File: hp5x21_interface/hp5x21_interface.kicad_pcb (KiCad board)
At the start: 2 copper layers, 4 parts, among them IC1 74LVC4245APW,118, IC2 74LVC4245APW,118, IC3 74LVC4245APW,118

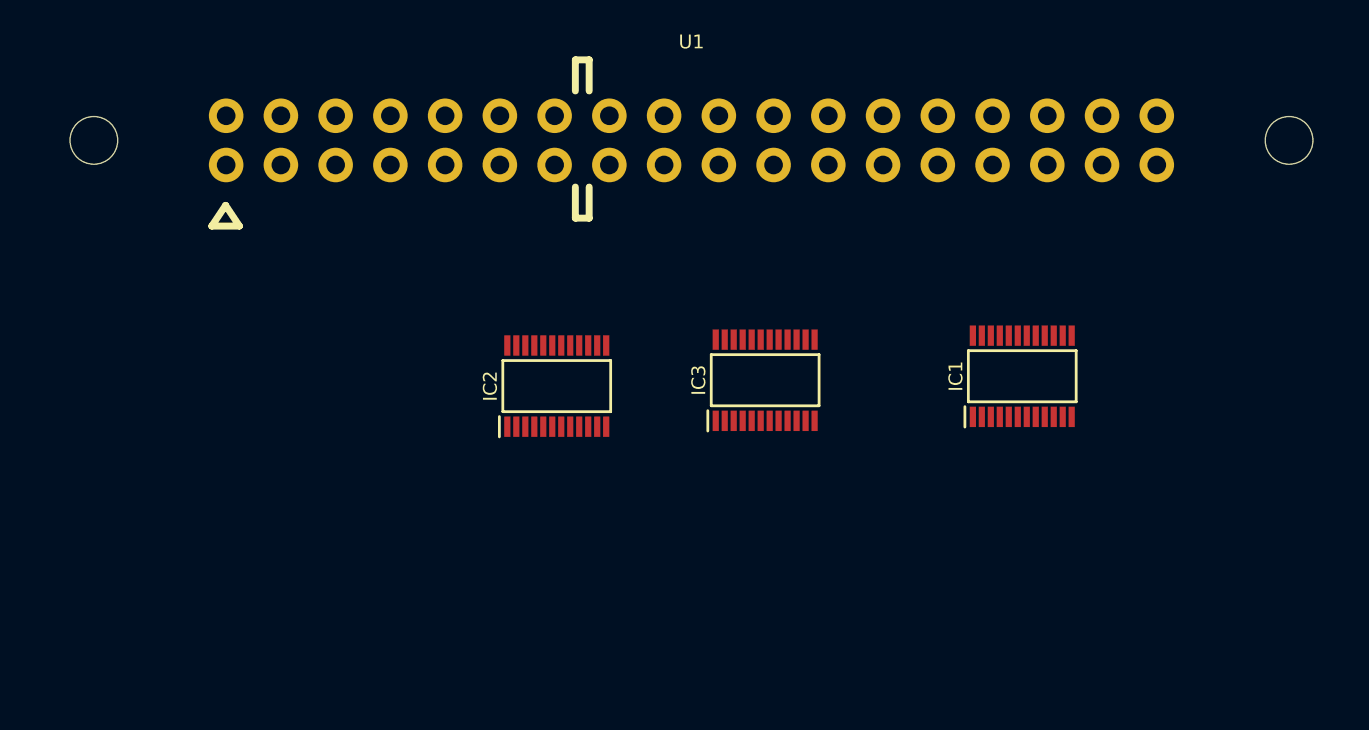
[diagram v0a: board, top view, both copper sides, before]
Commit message: Updated and released to JLCPCB
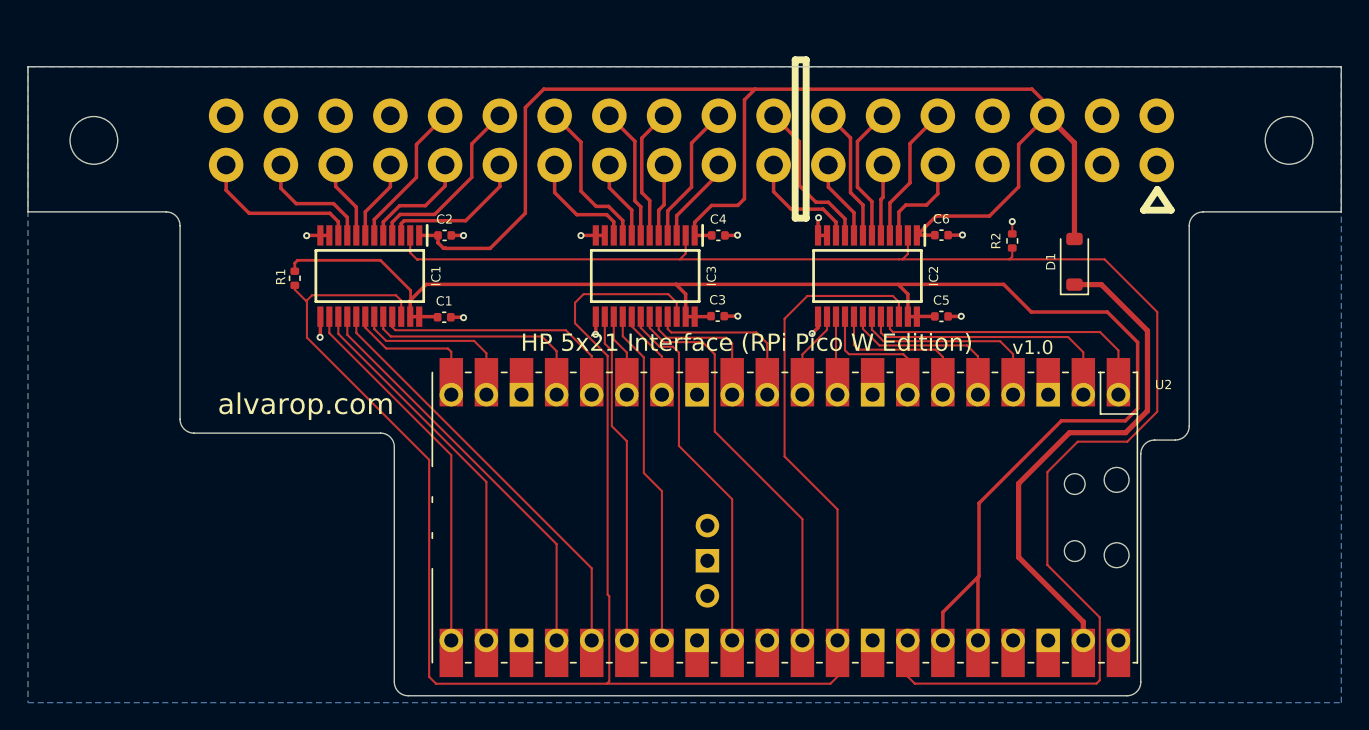
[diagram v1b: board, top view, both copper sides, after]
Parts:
- added C1: 0.1uF, Capacitor_SMD:C_0402_1005Metric, F.Cu at (120.1, 113.1)
- added C2: 0.1uF, Capacitor_SMD:C_0402_1005Metric, F.Cu at (120.1, 107.2)
- added C3: 0.1uF, Capacitor_SMD:C_0402_1005Metric, F.Cu at (139.9, 113.0)
- added C4: 0.1uF, Capacitor_SMD:C_0402_1005Metric, F.Cu at (139.9, 107.2)
- added C5: 0.1uF, Capacitor_SMD:C_0402_1005Metric, F.Cu at (156.1, 113.1)
- added C6: 0.1uF, Capacitor_SMD:C_0402_1005Metric, F.Cu at (156.1, 107.2)
- added D1: D_Schottky, Diode_SMD:D_SOD-123, F.Cu at (165.7, 109.1)
- added R1: 100k, Resistor_SMD:R_0402_1005Metric, F.Cu at (109.3, 110.3)
- added R2: 100k, Resistor_SMD:R_0402_1005Metric, F.Cu at (161.2, 107.6)
- added U2: PicoW, RP2040:RPi_PicoW_SMD_TH, F.Cu at (144.8, 127.6)
- U1: value ~ -> 307-036-520-201; moved to B.Cu
- moved IC1 47.8 mm to (114.7, 110.1), turned to -90 degrees
- moved IC2 23.8 mm to (150.7, 110.1), turned to -90 degrees
- moved IC3 11.5 mm to (134.7, 110.1), turned to -90 degrees
- turned U1 to 180 degrees
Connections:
- IC1 pad 1: unconnected-(IC1-VCC(A)-Pad1) -> +5V
- IC1 pad 10: unconnected-(IC1-A7-Pad10) -> /IO0_D
- IC1 pad 11: unconnected-(IC1-GND_1-Pad11) -> GND
- IC1 pad 12: unconnected-(IC1-GND_2-Pad12) -> GND
- IC1 pad 13: unconnected-(IC1-GND_3-Pad13) -> GND
- IC1 pad 14: /IO0_D -> /IO0_D_3V
- IC1 pad 15: /IO0_C -> /IO0_A_3V
- IC1 pad 16: /IO0_B -> /IO0_B_3V
- IC1 pad 17: /IO0_A -> /IO0_C_3V
- IC1 pad 18: /IO3_D -> /IO3_A_3V
- IC1 pad 19: /IO3_C -> /IO5_C_3V
- IC1 pad 2: unconnected-(IC1-DIR-Pad2) -> /DIR
- IC1 pad 20: /IO3_B -> /IO3_D_3V
- IC1 pad 21: /IO3_A -> /IO5_B_3V
- IC1 pad 22: unconnected-(IC1-~{OE}-Pad22) -> /~{OE}
- IC1 pad 23: unconnected-(IC1-VCC(B)_1-Pad23) -> +3.3V
- IC1 pad 24: unconnected-(IC1-VCC(B)_2-Pad24) -> +3.3V
- IC1 pad 3: unconnected-(IC1-A0-Pad3) -> /IO5_B
- IC1 pad 4: unconnected-(IC1-A1-Pad4) -> /IO3_D
- IC1 pad 5: unconnected-(IC1-A2-Pad5) -> /IO5_C
- IC1 pad 6: unconnected-(IC1-A3-Pad6) -> /IO3_A
- IC1 pad 7: unconnected-(IC1-A4-Pad7) -> /IO0_C
- IC1 pad 8: unconnected-(IC1-A5-Pad8) -> /IO0_B
- IC1 pad 9: unconnected-(IC1-A6-Pad9) -> /IO0_A
- IC2 pad 1: unconnected-(IC2-VCC(A)-Pad1) -> +5V
- IC2 pad 10: unconnected-(IC2-A7-Pad10) -> /IO1_C
- IC2 pad 11: unconnected-(IC2-GND_1-Pad11) -> GND
- IC2 pad 12: unconnected-(IC2-GND_2-Pad12) -> GND
- IC2 pad 13: unconnected-(IC2-GND_3-Pad13) -> GND
- IC2 pad 14: /IO2_D -> /IO1_C_3V
- IC2 pad 15: /IO2_C -> /IO2_C_3V
- IC2 pad 16: /IO2_B -> /IO1_B_3V
- IC2 pad 17: /IO2_A -> /IO2_B_3V
- IC2 pad 18: /IO1_D -> /IO2_A_3V
- IC2 pad 19: /IO1_C -> /IO1_A_3V
- IC2 pad 2: unconnected-(IC2-DIR-Pad2) -> /DIR
- IC2 pad 20: /IO1_B -> /IO2_D_3V
- IC2 pad 21: /IO1_A -> /IO1_D_3V
- IC2 pad 22: unconnected-(IC2-~{OE}-Pad22) -> /~{OE}
- IC2 pad 23: unconnected-(IC2-VCC(B)_1-Pad23) -> +3.3V
- IC2 pad 24: unconnected-(IC2-VCC(B)_2-Pad24) -> +3.3V
- IC2 pad 3: unconnected-(IC2-A0-Pad3) -> /IO1_D
- IC2 pad 4: unconnected-(IC2-A1-Pad4) -> /IO2_D
- IC2 pad 5: unconnected-(IC2-A2-Pad5) -> /IO1_A
- IC2 pad 6: unconnected-(IC2-A3-Pad6) -> /IO2_A
- IC2 pad 7: unconnected-(IC2-A4-Pad7) -> /IO2_B
- IC2 pad 8: unconnected-(IC2-A5-Pad8) -> /IO1_B
- IC2 pad 9: unconnected-(IC2-A6-Pad9) -> /IO2_C
- IC3 pad 1: unconnected-(IC3-VCC(A)-Pad1) -> +5V
- IC3 pad 10: unconnected-(IC3-A7-Pad10) -> /IO5_D
- IC3 pad 11: unconnected-(IC3-GND_1-Pad11) -> GND
- IC3 pad 12: unconnected-(IC3-GND_2-Pad12) -> GND
- IC3 pad 13: unconnected-(IC3-GND_3-Pad13) -> GND
- IC3 pad 14: /IO5_D -> /IO5_D_3V
- IC3 pad 15: /IO5_C -> /IO3_B_3V
- IC3 pad 16: /IO5_B -> /IO5_A_3V
- IC3 pad 17: /IO5_A -> /IO3_C_3V
- IC3 pad 18: /IO4_D -> /IO4_A_3V
- IC3 pad 19: /IO4_C -> /IO4_C_3V
- IC3 pad 2: unconnected-(IC3-DIR-Pad2) -> /DIR
- IC3 pad 20: /IO4_B -> /IO4_D_3V
- IC3 pad 21: /IO4_A -> /IO4_B_3V
- IC3 pad 22: unconnected-(IC3-~{OE}-Pad22) -> /~{OE}
- IC3 pad 23: unconnected-(IC3-VCC(B)_1-Pad23) -> +3.3V
- IC3 pad 24: unconnected-(IC3-VCC(B)_2-Pad24) -> +3.3V
- IC3 pad 3: unconnected-(IC3-A0-Pad3) -> /IO4_B
- IC3 pad 4: unconnected-(IC3-A1-Pad4) -> /IO4_D
- IC3 pad 5: unconnected-(IC3-A2-Pad5) -> /IO4_C
- IC3 pad 6: unconnected-(IC3-A3-Pad6) -> /IO4_A
- IC3 pad 7: unconnected-(IC3-A4-Pad7) -> /IO3_C
- IC3 pad 8: unconnected-(IC3-A5-Pad8) -> /IO5_A
- IC3 pad 9: unconnected-(IC3-A6-Pad9) -> /IO3_B
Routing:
- net /~{OE}: track 0.00 -> 145.9 mm
- net +3.3V: track 0.00 -> 112.5 mm
- net /DIR: track 0.00 -> 112.2 mm
- net +5V: track 0.00 -> 97.3 mm
- net Net-(D1-K): track 0.00 -> 37.2 mm
- net /IO0_C_3V: track 0.00 -> 30.5 mm
- net /IO0_B_3V: track 0.00 -> 29.7 mm
- net /IO4_C_3V: track 0.00 -> 29.6 mm
- net /IO0_A_3V: track 0.00 -> 27.9 mm
- net /IO0_D_3V: track 0.00 -> 27.1 mm
- net /IO4_A_3V: track 0.00 -> 26.7 mm
- net /IO5_A_3V: track 0.00 -> 24.6 mm
- net /IO5_D_3V: track 0.00 -> 24.1 mm
- net /IO1_D_3V: track 0.00 -> 21.3 mm
- net /IO2_D_3V: track 0.00 -> 19.5 mm
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- added copper zone on B.Cu, net GND
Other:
- board outline added: 95 x 45.5 mm
- board text added: "${COMPANY}"
- board text added: "${TITLE}"
- board text added: "v${REVISION}"
